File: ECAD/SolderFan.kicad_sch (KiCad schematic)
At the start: 6 parts, among them M1 Motor_DC

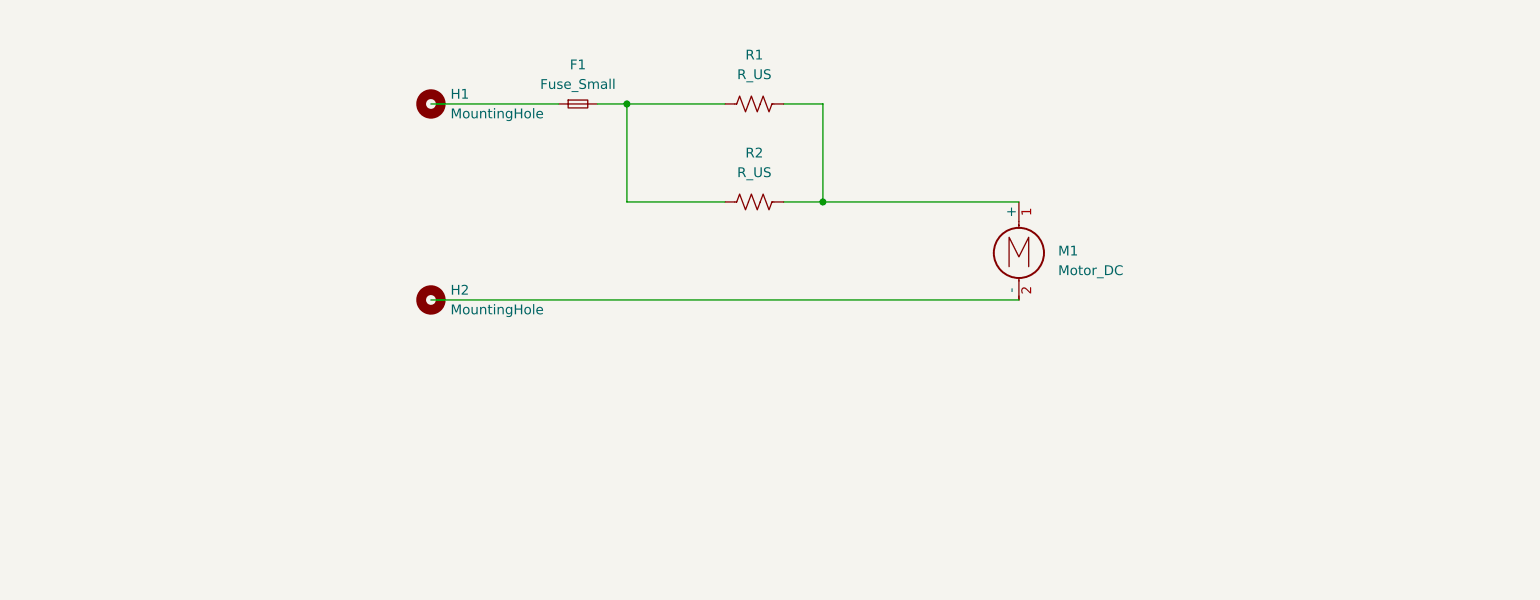
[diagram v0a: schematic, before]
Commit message: Updated Schematic, and PCB
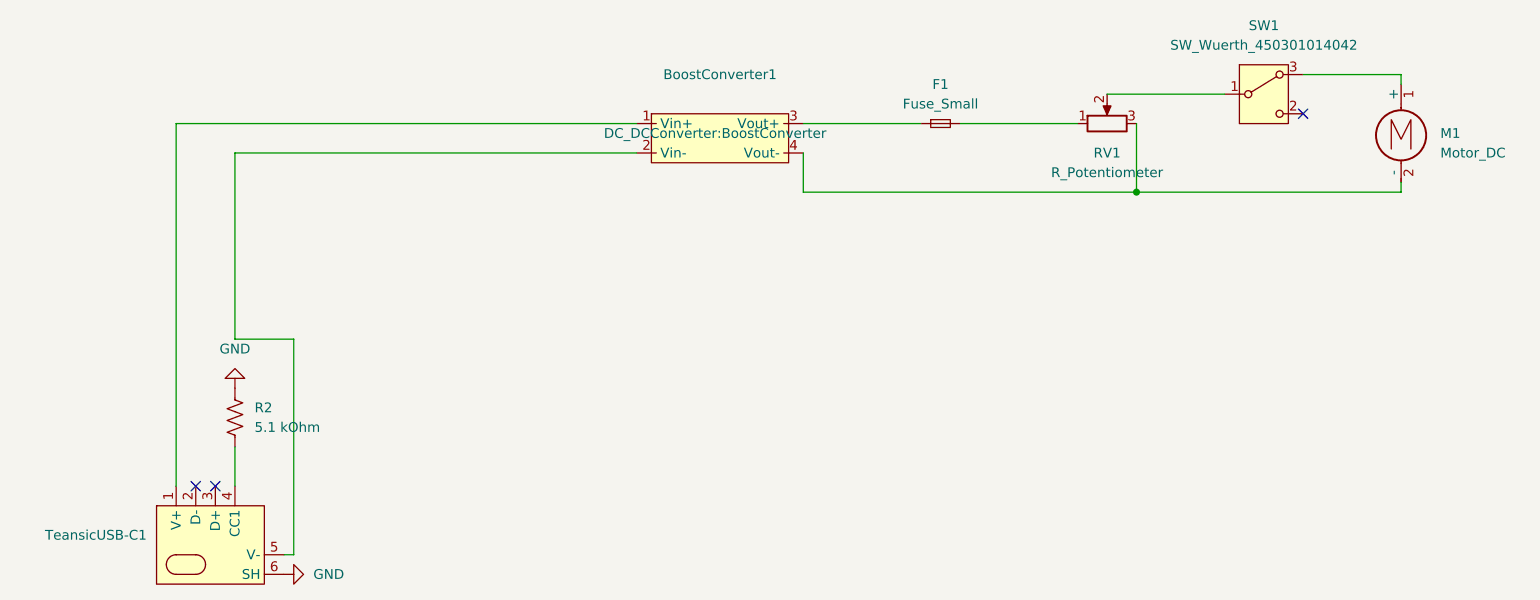
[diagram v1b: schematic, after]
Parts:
- removed H1, H2: MountingHole, symbol Mechanical:MountingHole
- removed R1: R_US, symbol Device:R_US
- added BoostConverter1: ~, DC_DCConverter:BoostConverter, symbol DC_DCConverters:BoostAdjustable
- added RV1: R_Potentiometer, Potentiometer_THT_Custom:Taiss3PTHTPot, symbol Device:R_Potentiometer
- added SW1: SW_Wuerth_450301014042, Button_Switch_THT:SW_Slide-03_Wuerth-WS-SLTV_10x2.5x6.4_P2.54mm, symbol Switch:SW_Wuerth_450301014042
- added TeansicUSB-C1: ~, USB_C_Connector_THT:TeansicUSB_C_6PIN, symbol Custom_Connectors:TeansicUSB-C
- F1: footprint (none) -> Fuse_Custom:BLX-A Fuse Holder
- M1: footprint (none) -> Connector_JST:JST_XH_B2B-XH-AM_1x02_P2.50mm_Vertical
- R2: value R_US -> 5.1 kOhm; footprint (none) -> Resistor_THT:R_Axial_DIN0204_L3.6mm_D1.6mm_P5.08mm_Horizontal
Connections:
- net at F1.1: now also BoostConverter1.3 (Vout+)
- net at F1.2: now also RV1.1; no longer R2.1
- net at M1.1 (+): now also SW1.3 (A); no longer R2.2
- net at M1.2 (-): now also BoostConverter1.4 (Vout-), RV1.3
- new net: RV1.2, SW1.1 (B)
- new net: BoostConverter1.1 (Vin+), TeansicUSB-C1.1 (V+)
- new net: BoostConverter1.2 (Vin-), TeansicUSB-C1.5 (V-)
- new net: R2.2, TeansicUSB-C1.4 (CC1)
- new net GND: R2.1, TeansicUSB-C1.6 (SH)
- no-connect marks 0 -> 3
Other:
- moved on the sheet: F1, M1
